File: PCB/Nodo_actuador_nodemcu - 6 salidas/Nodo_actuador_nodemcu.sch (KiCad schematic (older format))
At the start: 10 parts, among them J1 Entrada 5V, J2 Conector botones, J3 Conector_reles, U1 NodeMCU_Amica_R2

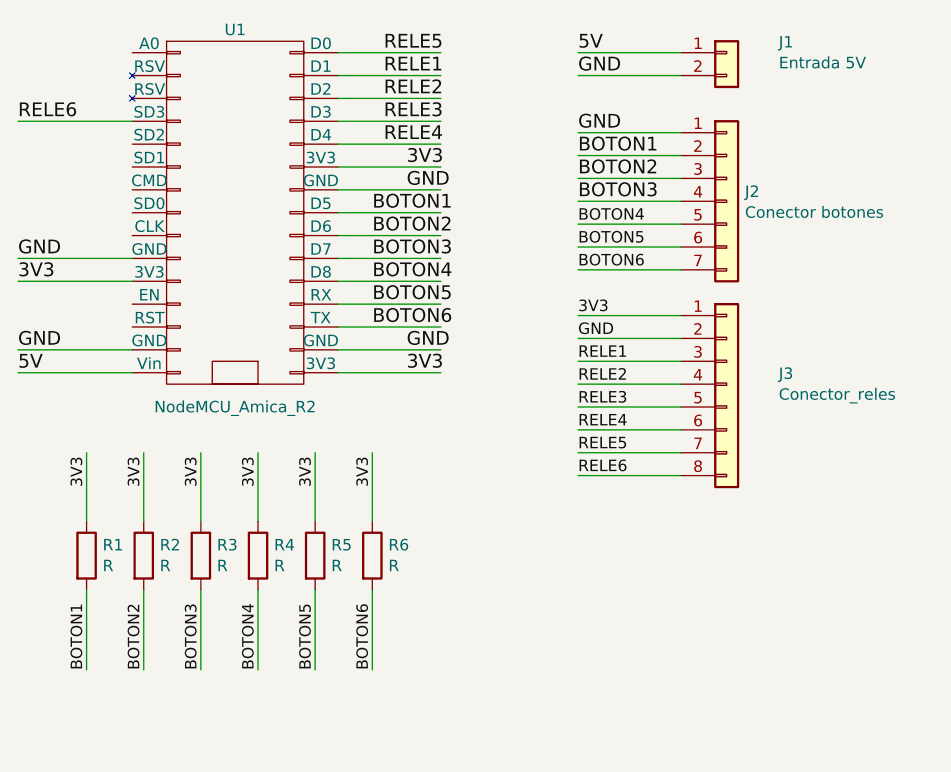
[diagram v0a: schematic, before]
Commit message: pcb
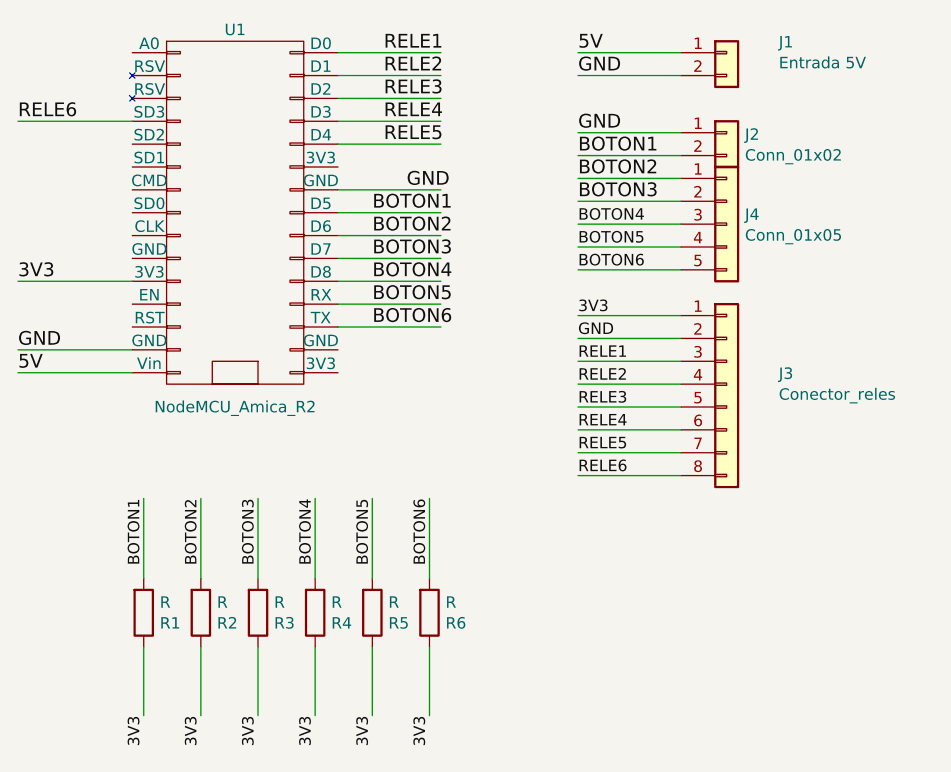
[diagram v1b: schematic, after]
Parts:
- removed J2: Conector botones, symbol Connector_Generic:Conn_01x07
- added J2: Conn_01x02, TerminalBlock:TerminalBlock_bornier-2_P5.08mm, symbol Connector_Generic:Conn_01x02
- added J4: Conn_01x05, TerminalBlock:TerminalBlock_bornier-5_P5.08mm, symbol Connector_Generic:Conn_01x05
- J1: footprint (none) -> TerminalBlock:TerminalBlock_bornier-2_P5.08mm
- J3: footprint (none) -> Connector_PinSocket_2.54mm:PinSocket_1x08_P2.54mm_Vertical
- R1, R2, R3, R4, R5, R6: footprint (none) -> Resistor_THT:R_Axial_DIN0207_L6.3mm_D2.5mm_P7.62mm_Horizontal
- U1: footprint (none) -> nodemcu:NodeMCU_Amica_R2
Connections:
- wire segments 49 -> 45
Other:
- moved on the sheet: R1, R2, R3, R4, R5, R6
